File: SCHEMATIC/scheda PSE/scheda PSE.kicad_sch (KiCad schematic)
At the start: 4 parts

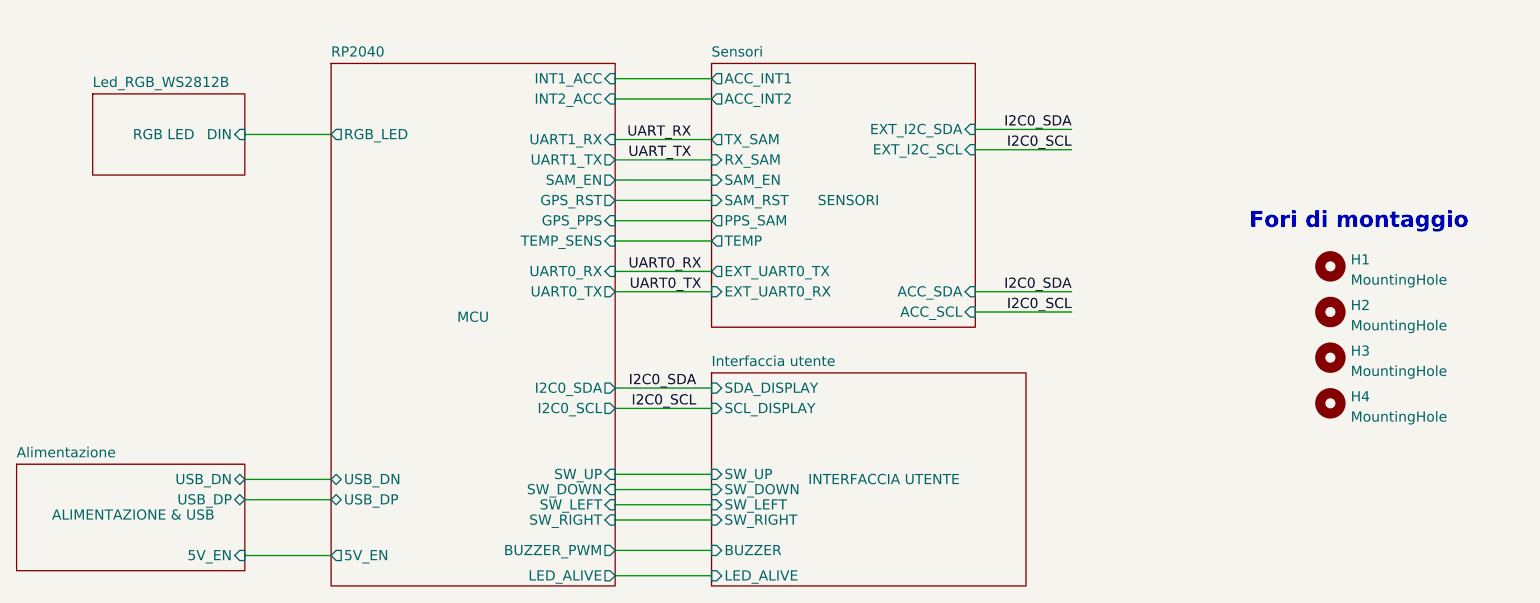
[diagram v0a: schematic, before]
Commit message: finito lo sbroglio (magari da ricontrollare)
finito lo sbroglio, controllato già io ma meglio ridare una controllata.
Da sistemare tutta la serigrafia
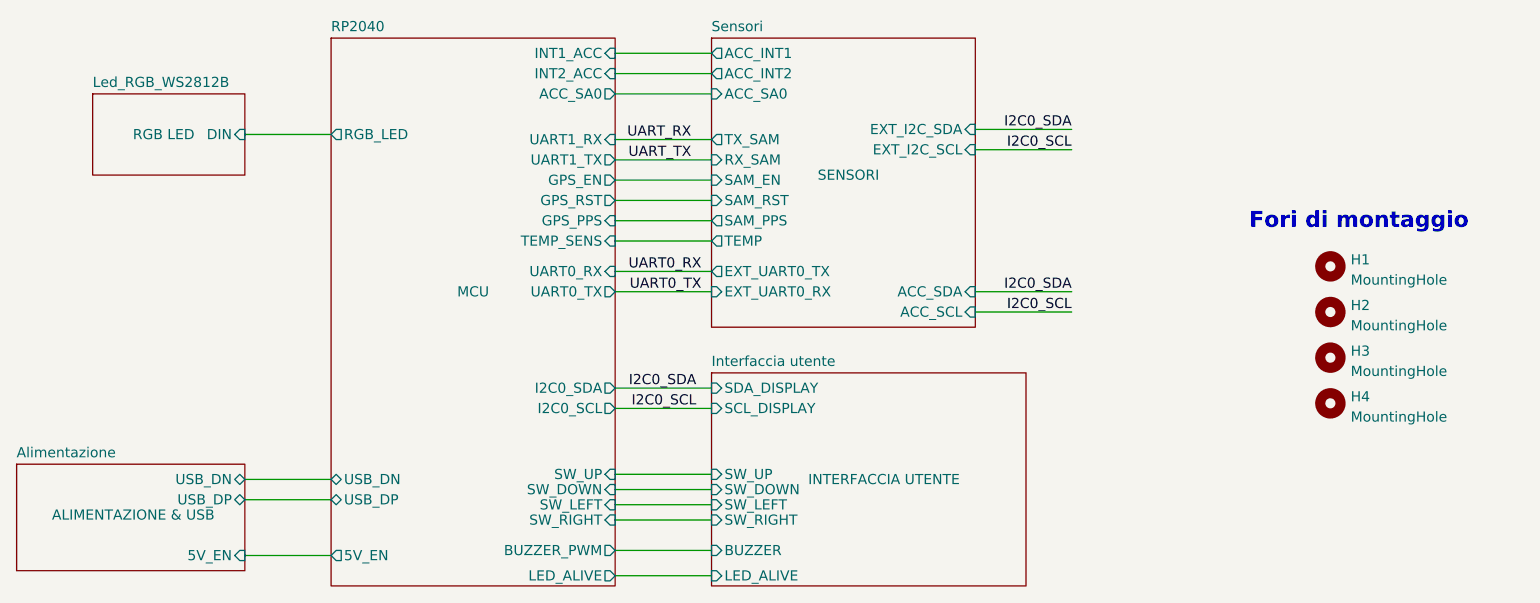
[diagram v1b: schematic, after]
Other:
- sheet RP2040 ports: added ACC_SA0, GPS_EN; removed SAM_EN
- sheet Sensori ports: added ACC_SA0, SAM_PPS; removed PPS_SAM
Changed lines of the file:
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@@
     (stroke (width 0) (type default) (color 0 0 0 0))
   )
-  (wire (pts (xy 149.86 69.85) (xy 161.925 69.85))
+  (wire (pts (xy 149.86 66.675) (xy 161.925 66.675))
     (stroke (width 0) (type default) (color 0 0 0 0))
   )
@@
     (stroke (width 0) (type default) (color 0 0 0 0))
   )
+  (wire (pts (xy 149.86 69.215) (xy 161.925 69.215))
+    (stroke (width 0) (type default) (color 0 0 0 0))
+  )
   (wire (pts (xy 149.86 106.045) (xy 161.925 106.045))
     (stroke (width 0) (type default) (color 0 0 0 0))
@@
     (stroke (width 0) (type default) (color 0 0 0 0))
   )
-  (wire (pts (xy 149.86 67.31) (xy 161.925 67.31))
+  (wire (pts (xy 149.86 64.135) (xy 161.925 64.135))
     (stroke (width 0) (type default) (color 0 0 0 0))
   )
@@
     )
   )
-  (sheet (at 161.925 65.405) (size 33.02 33.02)
+  (sheet (at 161.925 62.23) (size 33.02 36.195)
     (stroke (width 0.1524) (type solid) (color 0 0 0 0))
     (fill (color 0 0 0 0.0000))
-    (property "Sheet name" "Sensori" (id 0) (at 161.925 64.6934 0)
+    (property "Sheet name" "Sensori" (id 0) (at 161.925 61.5184 0)
       (effects (font (size 1.27 1.27)) (justify left bottom))
     )
-    (property "Sheet file" "sensori.kicad_sch" (id 1) (at 161.925 92.71 0)
+    (property "Sheet file" "sensori.kicad_sch" (id 1) (at 161.925 89.535 0)
       (effects (font (size 1.27 1.27)) (justify left top) hide)
     )
-    (property "Etichetta" "SENSORI" (id 2) (at 179.07 82.55 0))
+    (property "Etichetta" "SENSORI" (id 2) (at 179.07 79.375 0))
     (pin "TX_SAM" output (at 161.925 74.93 180)
       (effects (font (size 1.27 1.27)) (justify left))
@@
       (effects (font (size 1.27 1.27)) (justify left))
     )
-    (pin "ACC_INT2" output (at 161.925 69.85 180)
-      (effects (font (size 1.27 1.27)) (justify left))
-    )
-    (pin "ACC_INT1" output (at 161.925 67.31 180)
+    (pin "ACC_INT2" output (at 161.925 66.675 180)
+      (effects (font (size 1.27 1.27)) (justify left))
+    )
+    (pin "ACC_INT1" output (at 161.925 64.135 180)
       (effects (font (size 1.27 1.27)) (justify left))
     )
@@
       (effects (font (size 1.27 1.27)) (justify left))
     )
-    (pin "PPS_SAM" output (at 161.925 85.09 180)
+    (pin "SAM_PPS" output (at 161.925 85.09 180)
+      (effects (font (size 1.27 1.27)) (justify left))
+    )
+    (pin "ACC_SA0" input (at 161.925 69.215 180)
       (effects (font (size 1.27 1.27)) (justify left))
     )
@@
     )
   )
-  (sheet (at 114.3 65.405) (size 35.56 65.405)
+  (sheet (at 114.3 62.23) (size 35.56 68.58)
     (stroke (width 0.1524) (type solid) (color 0 0 0 0))
     (fill (color 0 0 0 0.0000))
-    (property "Sheet name" "RP2040" (id 0) (at 114.3 64.6934 0)
+    (property "Sheet name" "RP2040" (id 0) (at 114.3 61.5184 0)
       (effects (font (size 1.27 1.27)) (justify left bottom))
     )
-    (property "Sheet file" "rp2040.kicad_sch" (id 1) (at 114.3 131.3946 0)
+    (property "Sheet file" "rp2040.kicad_sch" (id 1) (at 114.3 128.2196 0)
       (effects (font (size 1.27 1.27)) (justify left top) hide)
     )
-    (property "Etichetta" "MCU" (id 2) (at 132.08 97.155 0))
+    (property "Etichetta" "MCU" (id 2) (at 132.08 93.98 0))
     (pin "USB_DN" bidirectional (at 114.3 117.475 180)
       (effects (font (size 1.27 1.27)) (justify left))
@@
       (effects (font (size 1.27 1.27)) (justify left))
     )
-    (pin "INT1_ACC" input (at 149.86 67.31 0)
-      (effects (font (size 1.27 1.27)) (justify right))
-    )
-    (pin "INT2_ACC" input (at 149.86 69.85 0)
+    (pin "INT1_ACC" input (at 149.86 64.135 0)
+      (effects (font (size 1.27 1.27)) (justify right))
+    )
+    (pin "INT2_ACC" input (at 149.86 66.675 0)
       (effects (font (size 1.27 1.27)) (justify right))
     )
@@
       (effects (font (size 1.27 1.27)) (justify right))
     )
-    (pin "SAM_EN" output (at 149.86 80.01 0)
-      (effects (font (size 1.27 1.27)) (justify right))
-    )
     (pin "GPS_RST" output (at 149.86 82.55 0)
       (effects (font (size 1.27 1.27)) (justify right))
     )
     (pin "GPS_PPS" input (at 149.86 85.09 0)
+      (effects (font (size 1.27 1.27)) (justify right))
+    )
+    (pin "ACC_SA0" output (at 149.86 69.215 0)
+      (effects (font (size 1.27 1.27)) (justify right))
+    )
+    (pin "GPS_EN" output (at 149.86 80.01 0)
       (effects (font (size 1.27 1.27)) (justify right))
     )
@@
       (reference "#PWR078") (unit 1) (value "GND") (footprint "")
     )
-    (path "/7389e30f-cc4a-4964-bca3-cd95052ca62a/028caaaa-a788-48f0-8e29-0eb2d6869e1a"
-      (reference "#PWR079") (unit 1) (value "GND") (footprint "")
-    )
     (path "/7389e30f-cc4a-4964-bca3-cd95052ca62a/aa1b72ec-e86b-4492-ab96-18057e24a375"
